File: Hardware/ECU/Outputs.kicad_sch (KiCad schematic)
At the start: 25 parts, among them IC2 ZXMS6006DT8, IC3 ZXMS6006DT8, IC4 ZXMS6006DT8

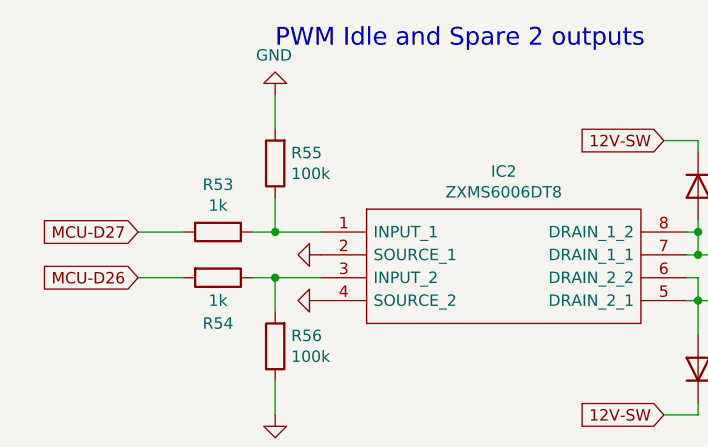
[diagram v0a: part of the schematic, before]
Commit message: PCB
Platine Vernetzt
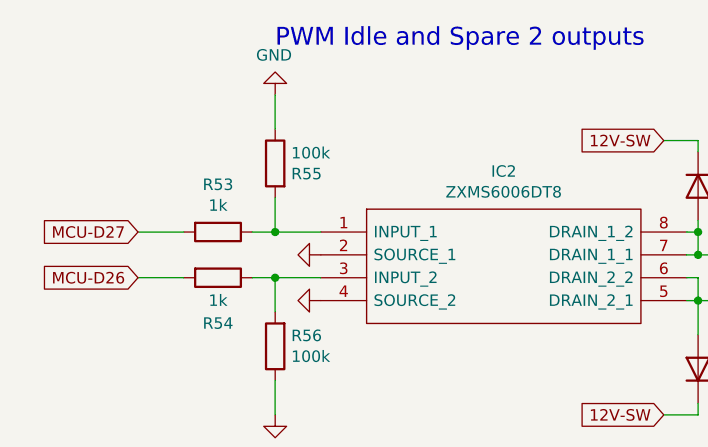
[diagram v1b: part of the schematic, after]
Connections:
- net GND: now also R55.1; no longer R55.2
- net at IC2.1 (INPUT_1), R53.1: now also R55.2; no longer R55.1
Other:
- moved on the sheet: R55
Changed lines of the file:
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@@
 	(symbol
 		(lib_id "Device:R")
-		(at 48.26 36.83 180)
+		(at 48.26 36.83 0)
+		(mirror y)
 		(unit 1)
 		(exclude_from_sim no)
@@
 		(dnp no)
 		(property "Reference" "R55"
-			(at 50.038 35.6616 0)
+			(at 50.038 37.9984 0)
 			(effects
 				(font
@@
 		)
 		(property "Value" "100k"
-			(at 50.038 37.973 0)
+			(at 50.038 35.687 0)
 			(effects
 				(font
@@
 		)
 		(property "Manufacturer_Name" "Yageo"
-			(at 99.06 1.27 0)
+			(at 99.06 72.39 0)
 			(effects
 				(font
@@
 		)
 		(property "Manufacturer_Part_Number" "RC0805FR-07100KL"
-			(at 99.06 1.27 0)
+			(at 99.06 72.39 0)
 			(effects
 				(font
@@
 		)
 		(property "URL" "https://www.digikey.com/product-detail/en/yageo/RC0805FR-07100KL/311-100KCRCT-ND/730491"
-			(at 99.06 1.27 0)
+			(at 99.06 72.39 0)
 			(effects
 				(font
@@
 		)
 		(property "Digikey Part Number" "311-100KCRCT-ND"
-			(at 99.06 1.27 0)
+			(at 99.06 72.39 0)
 			(effects
 				(font
